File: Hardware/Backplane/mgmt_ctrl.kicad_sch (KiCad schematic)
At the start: 20 parts, among them J501 Conn_01x03, Q501 S3134K, U502 CH32V003FxPx, U503 NL17SZS11DFT2G-Q

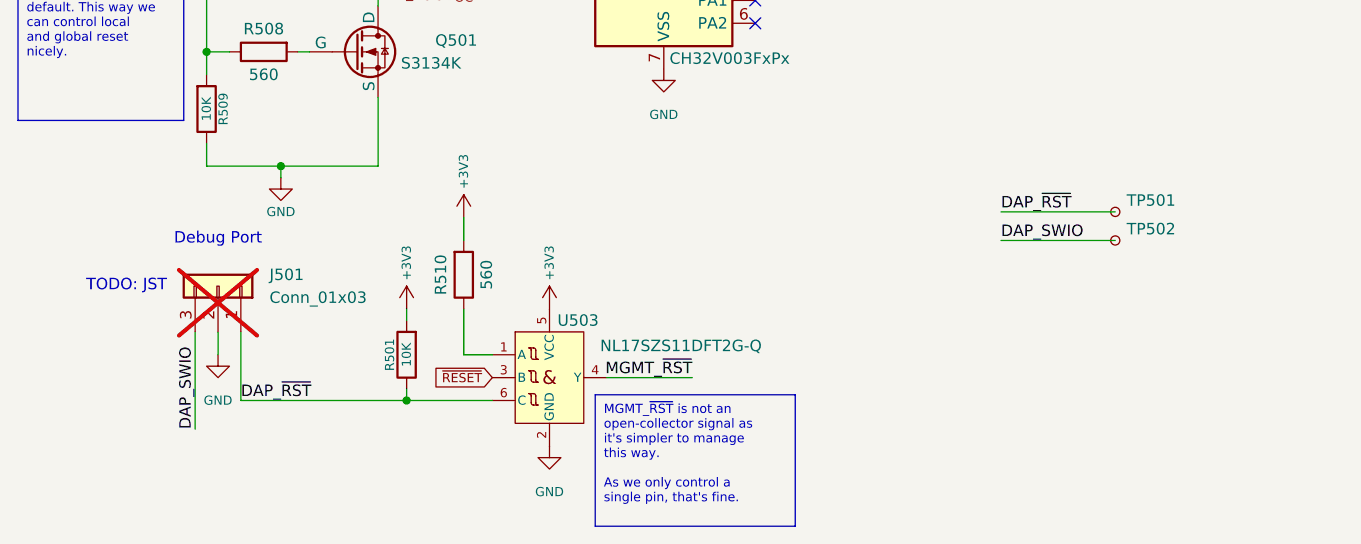
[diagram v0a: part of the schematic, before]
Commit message: Further backplane PCB cleanup.
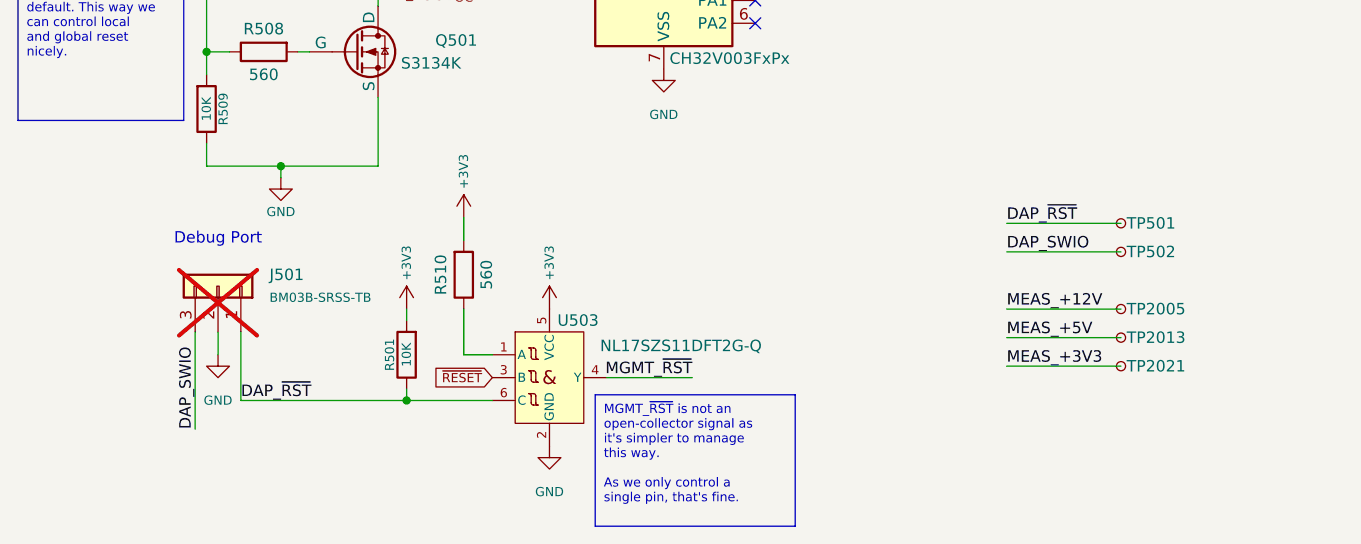
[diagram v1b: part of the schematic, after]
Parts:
- added TP2005, TP2013, TP2021: TestPoint_Small, TestPoint:TestPoint_Pad_D1.0mm, symbol Connector:TestPoint_Small
- J501: value Conn_01x03 -> BM03B-SRSS-TB; footprint Connector_Molex:Molex_PicoBlade_53047-0310_1x03_P1.25mm_Vertical -> Connector_JST:JST_SH_BM03B-SRSS-TB_1x03-1MP_P1.00mm_Vertical; Digikey Part No WM1732-ND -> 455-BM03B-SRSS-TBTR-ND
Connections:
- net MEAS_+12V: now also TP2005.1
- net MEAS_+3V3: now also TP2021.1
- net MEAS_+5V: now also TP2013.1
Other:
- note removed: "TODO: JST"
- moved on the sheet: TP501, TP502
